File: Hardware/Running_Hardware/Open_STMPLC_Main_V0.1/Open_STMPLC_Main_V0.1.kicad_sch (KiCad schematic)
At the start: 4 parts

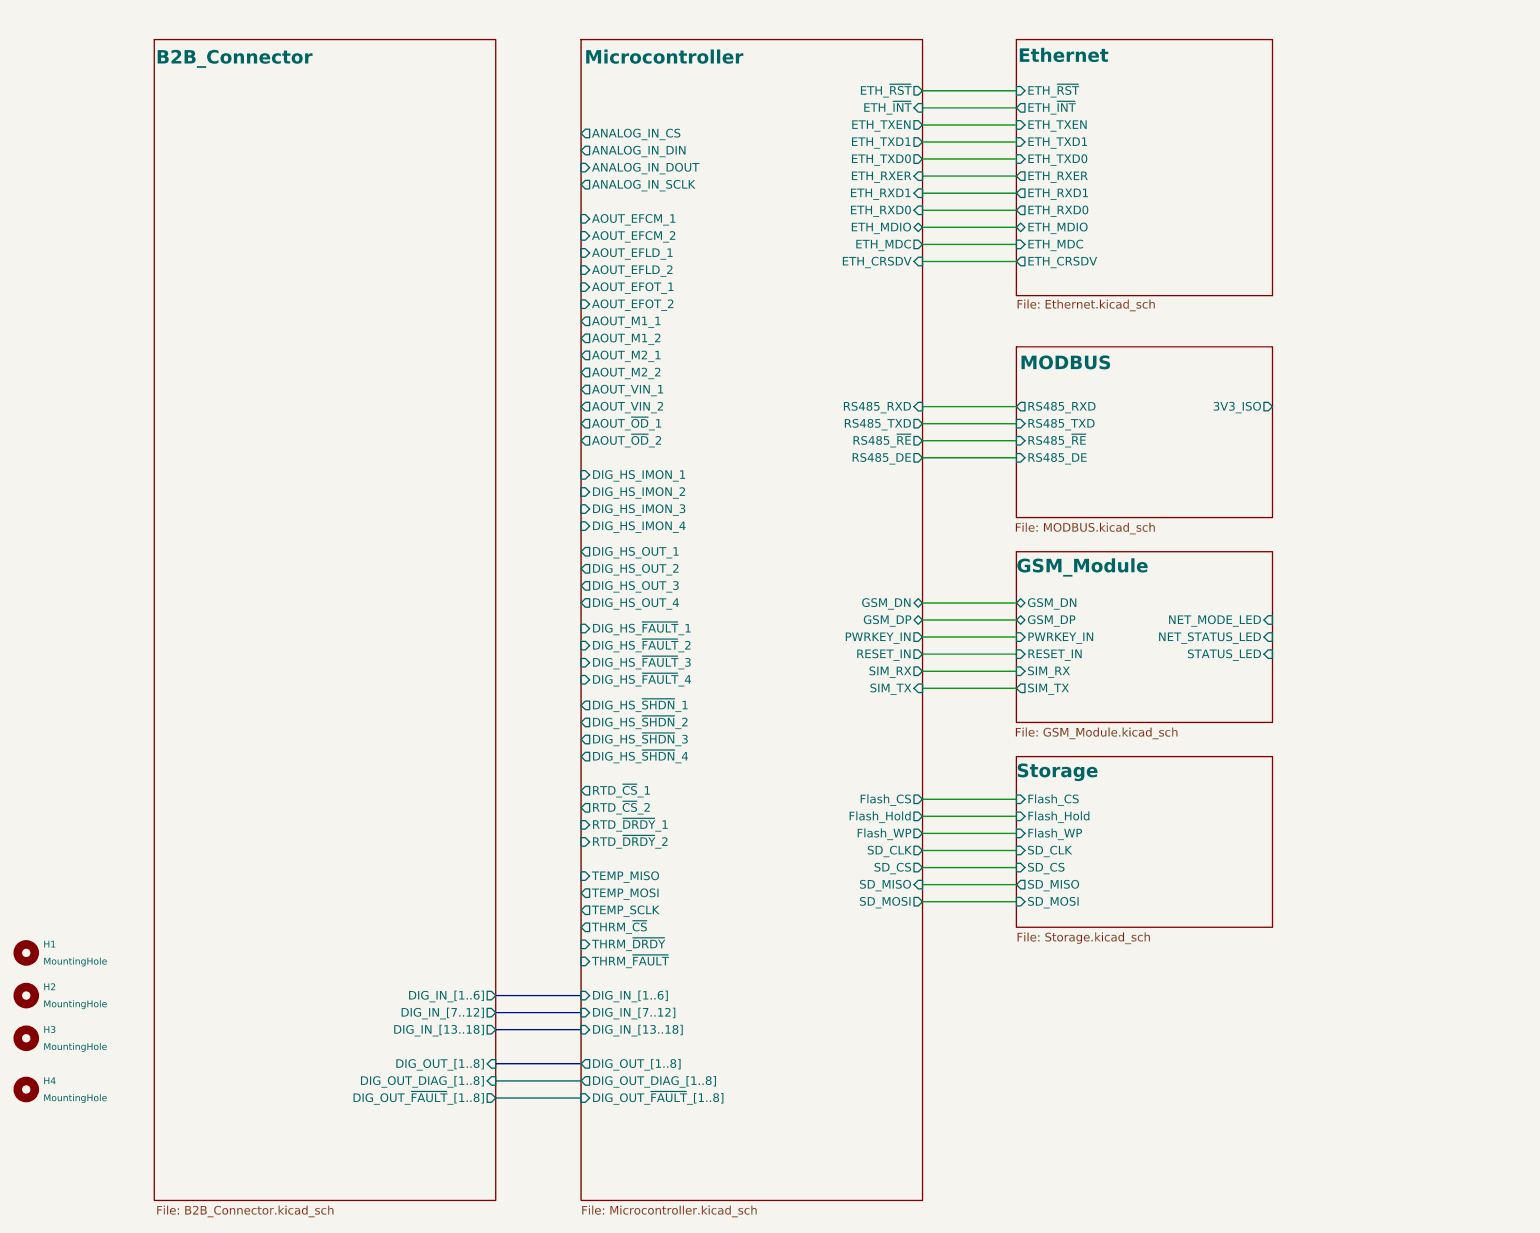
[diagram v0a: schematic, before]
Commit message: Main PCB changes
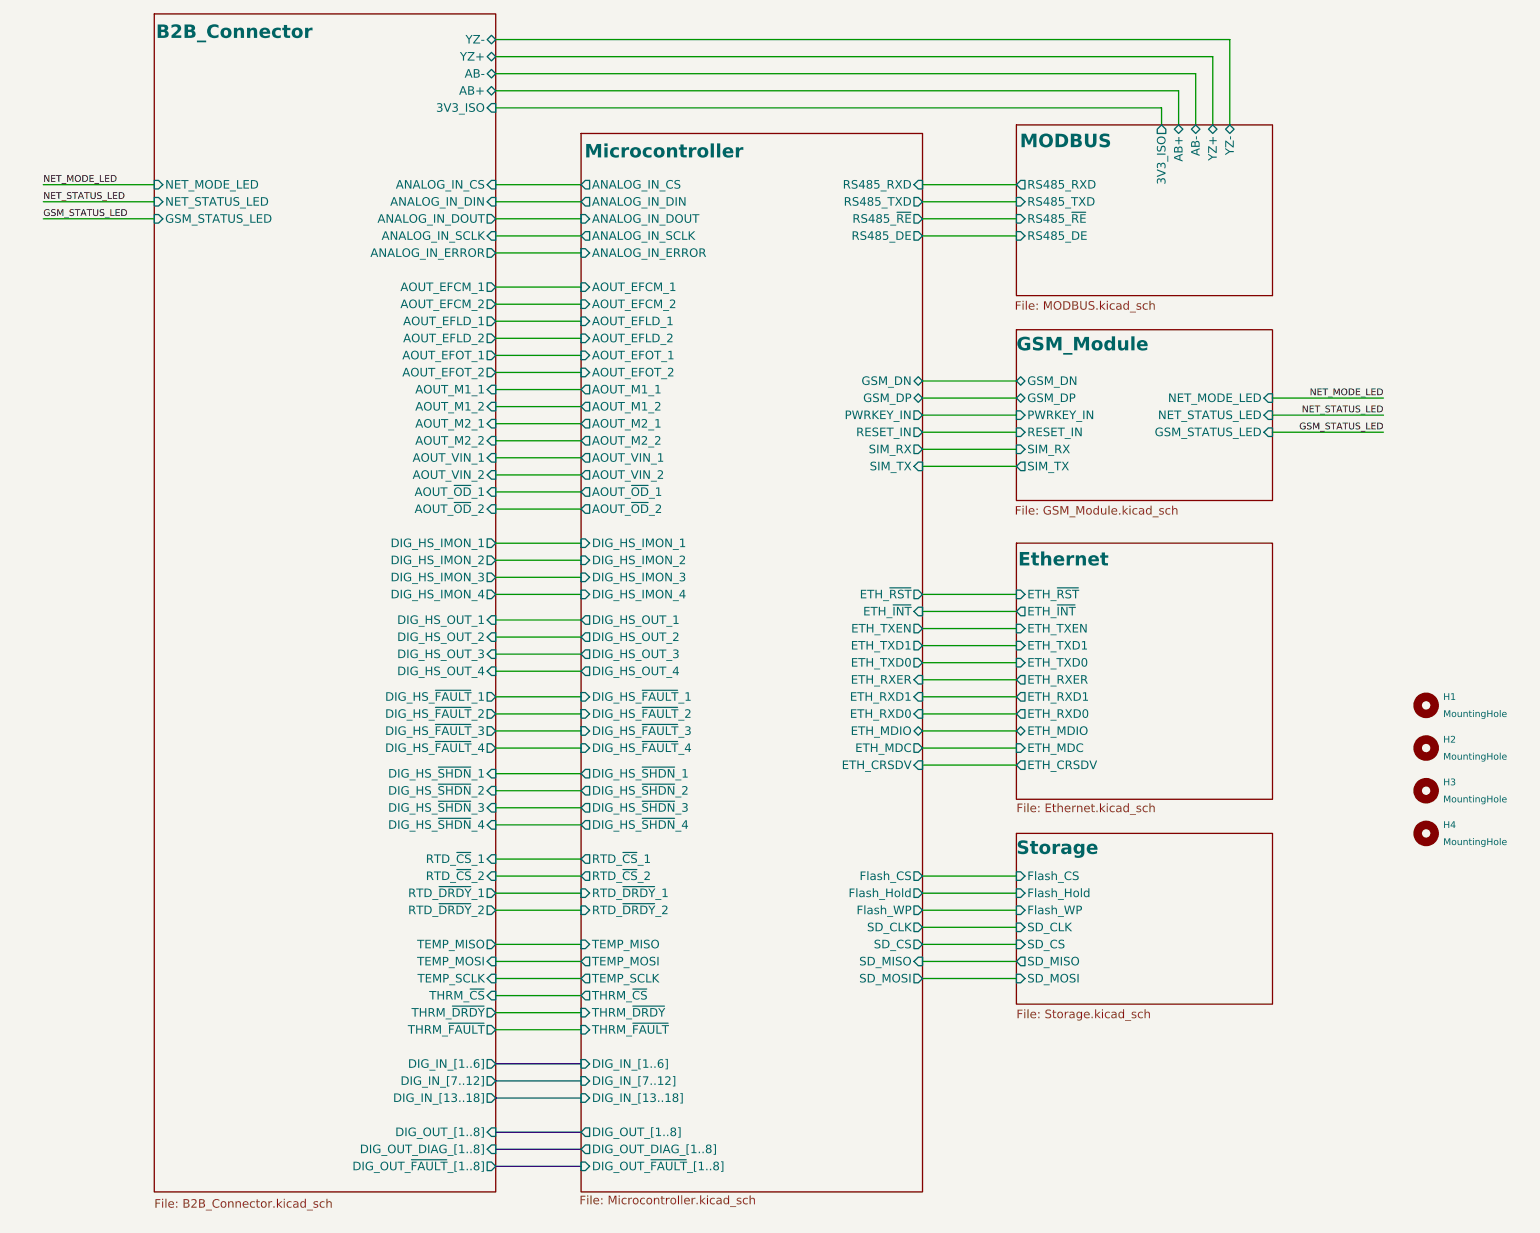
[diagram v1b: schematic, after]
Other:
- sheet B2B_Connector ports: added 3V3_ISO, AB+, AB-, ANALOG_IN_CS, ANALOG_IN_DIN, ANALOG_IN_DOUT, ANALOG_IN_ERROR, ANALOG_IN_SCLK, AOUT_EFCM_1, AOUT_EFCM_2, AOUT_EFLD_1, AOUT_EFLD_2, AOUT_EFOT_1, AOUT_EFOT_2, AOUT_M1_1, AOUT_M1_2, AOUT_M2_1, AOUT_M2_2, AOUT_VIN_1, AOUT_VIN_2, AOUT_~{OD}_1, AOUT_~{OD}_2, DIG_HS_IMON_1, DIG_HS_IMON_2, DIG_HS_IMON_3, DIG_HS_IMON_4, DIG_HS_OUT_1, DIG_HS_OUT_2, DIG_HS_OUT_3, DIG_HS_OUT_4, DIG_HS_~{FAULT}_1, DIG_HS_~{FAULT}_2, DIG_HS_~{FAULT}_3, DIG_HS_~{FAULT}_4, DIG_HS_~{SHDN}_1, DIG_HS_~{SHDN}_2, DIG_HS_~{SHDN}_3, DIG_HS_~{SHDN}_4, GSM_STATUS_LED, NET_MODE_LED, NET_STATUS_LED, RTD_~{CS}_1, RTD_~{CS}_2, RTD_~{DRDY}_1, RTD_~{DRDY}_2, TEMP_MISO, TEMP_MOSI, TEMP_SCLK, THRM_~{CS}, THRM_~{DRDY}, THRM_~{FAULT}, YZ+, YZ-; removed none
- sheet GSM_Module ports: added GSM_STATUS_LED; removed STATUS_LED
- sheet MODBUS ports: added AB+, AB-, YZ+, YZ-; removed none
- sheet Microcontroller ports: added ANALOG_IN_ERROR; removed none
- moved on the sheet: H1, H2, H3, H4
